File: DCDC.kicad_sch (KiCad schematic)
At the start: 23 parts, among them U11 LM76005RNPR

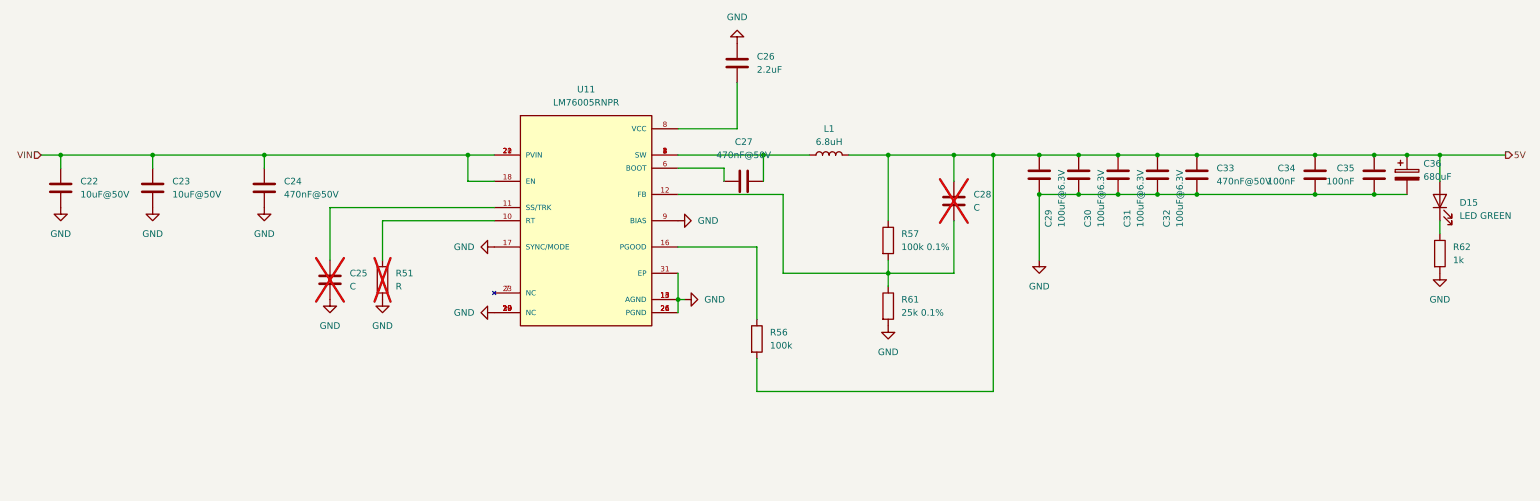
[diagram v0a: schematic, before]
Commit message: wip
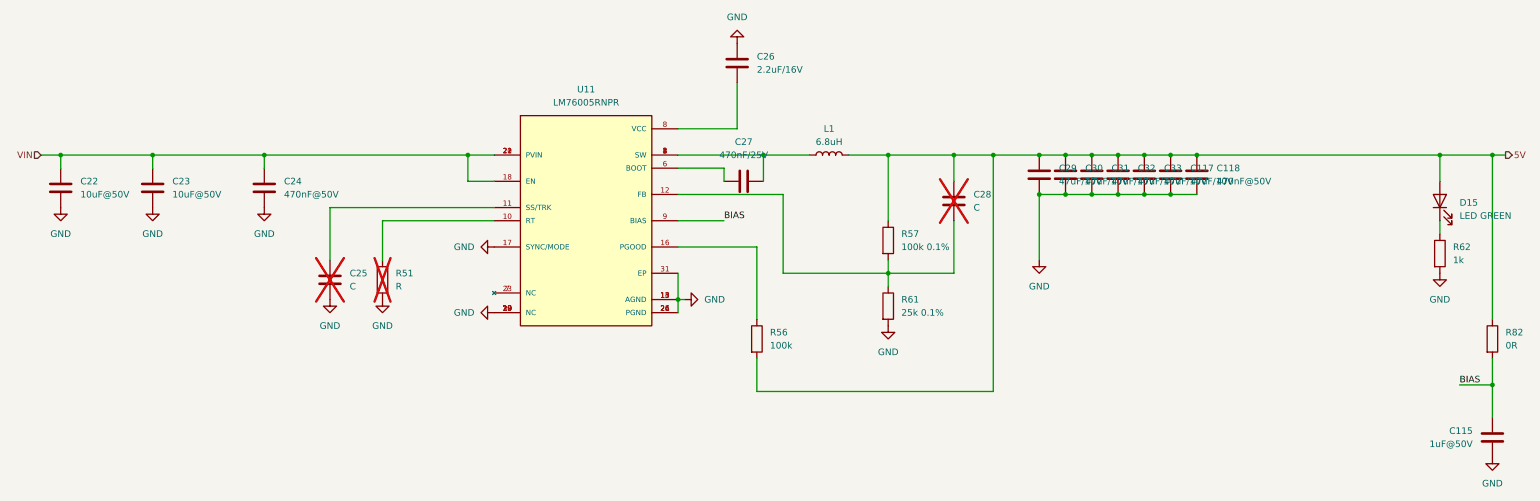
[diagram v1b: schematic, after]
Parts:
- removed C34, C35: 100nF, Capacitor_SMD:C_0402_1005Metric, symbol Device:C
- removed C36: 680uF, Capacitor_SMD:CP_Elec_10x12.5, symbol Device:C_Polarized
- added C115: 1uF@50V, Capacitor_SMD:C_0603_1608Metric, symbol Device:C
- added C117: 47uF/10V, Capacitor_SMD:C_1206_3216Metric, symbol Device:C
- added C118: 470nF@50V, Capacitor_SMD:C_0805_2012Metric, symbol Device:C
- added R82: 0R, Resistor_SMD:R_0603_1608Metric, symbol Device:R
- C25, C28: footprint Capacitor_SMD:C_0805_2012Metric -> Capacitor_SMD:C_0603_1608Metric
- C26: value 2.2uF -> 2.2uF/16V; footprint Capacitor_SMD:C_0805_2012Metric -> Capacitor_SMD:C_0603_1608Metric; JLC C377773 -> C23630
- C27: value 470nF@50V -> 470nF/25V; footprint Capacitor_SMD:C_0805_2012Metric -> Capacitor_SMD:C_0603_1608Metric; JLC C13967 -> C1623
- C29, C30, C31, C32: value 100uF@6.3V -> 47uF/10V; JLC C15008 -> C96123
- C33: value 470nF@50V -> 47uF/10V; footprint Capacitor_SMD:C_0805_2012Metric -> Capacitor_SMD:C_1206_3216Metric; JLC C13967 -> C96123
- R51: footprint Resistor_SMD:R_0805_2012Metric -> Resistor_SMD:R_0603_1608Metric
- R56: footprint Resistor_SMD:R_0805_2012Metric -> Resistor_SMD:R_0603_1608Metric; JLC C149504 -> C25803
- R57: footprint Resistor_SMD:R_0805_2012Metric -> Resistor_SMD:R_0603_1608Metric; JLC C149504 -> C122538
- R61: footprint Resistor_SMD:R_0805_2012Metric -> Resistor_SMD:R_0603_1608Metric; JLC C153306 -> C2828637
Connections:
- net 5V: now also C117.1, C118.1, R82.1
- net GND: now also C115.1, C117.2, C118.2; no longer U11.9 (BIAS)
- new net BIAS: C115.2, R82.2, U11.9 (BIAS)
